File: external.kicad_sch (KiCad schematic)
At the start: 47 parts, among them J5 Keyboard Connector, J6 Joystick 1, J7 Joystick 2, Q7 BC547B, Q8 BC547B, U66 SN74ALS175N (КР1533ТМ8), U67 8282 (КР580ИР82), U68 КР556РТ2, U72 КР556РТ2, U73 SN74ALS08 (КР1533ЛИ1), U74 SN74ALS08 (КР1533ЛИ1)

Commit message: Version 1.0 schematics and PCB complete
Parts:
- D1, D10, D14, D15, D16, D17, D18, D19, D2, D20, D21, D22, D23, D24, D25, D26, D27, D28, D29, D3, D4, D5, D6, D7, D8, D9: symbol Device:D -> Delta_s_m_Lib:D
- DA1: symbol Device:R_Network09 -> Delta_s_m_Lib:R_Network09
- J5: symbol Connector_Generic:Conn_02x12_Odd_Even -> Delta_s_m_Lib:Conn_02x12_Odd_Even
- J6, J7: symbol Connector:DIN-7 -> Delta_s_m_Lib:DIN-7
- Q7, Q8: symbol Transistor_BJT:BC547 -> Delta_s_m_Lib:BC547
- R50, R51, R52, R54, R55, R56, R57, R58, R59: symbol Device:R -> Delta_s_m_Lib:R
- U66: symbol 74xx:74LS175 -> Delta_s_m_Lib:74LS175
- U67: symbol w_connectors:8282 (КР580ИР82) -> Delta_s_m_Lib:8282 (КР580ИР82)
- U68, U72: symbol w_connectors:КР556РТ2 -> Delta_s_m_Lib:КР556РТ2
- U73, U74: symbol 74xx:74LS08 -> Delta_s_m_Lib:74LS08

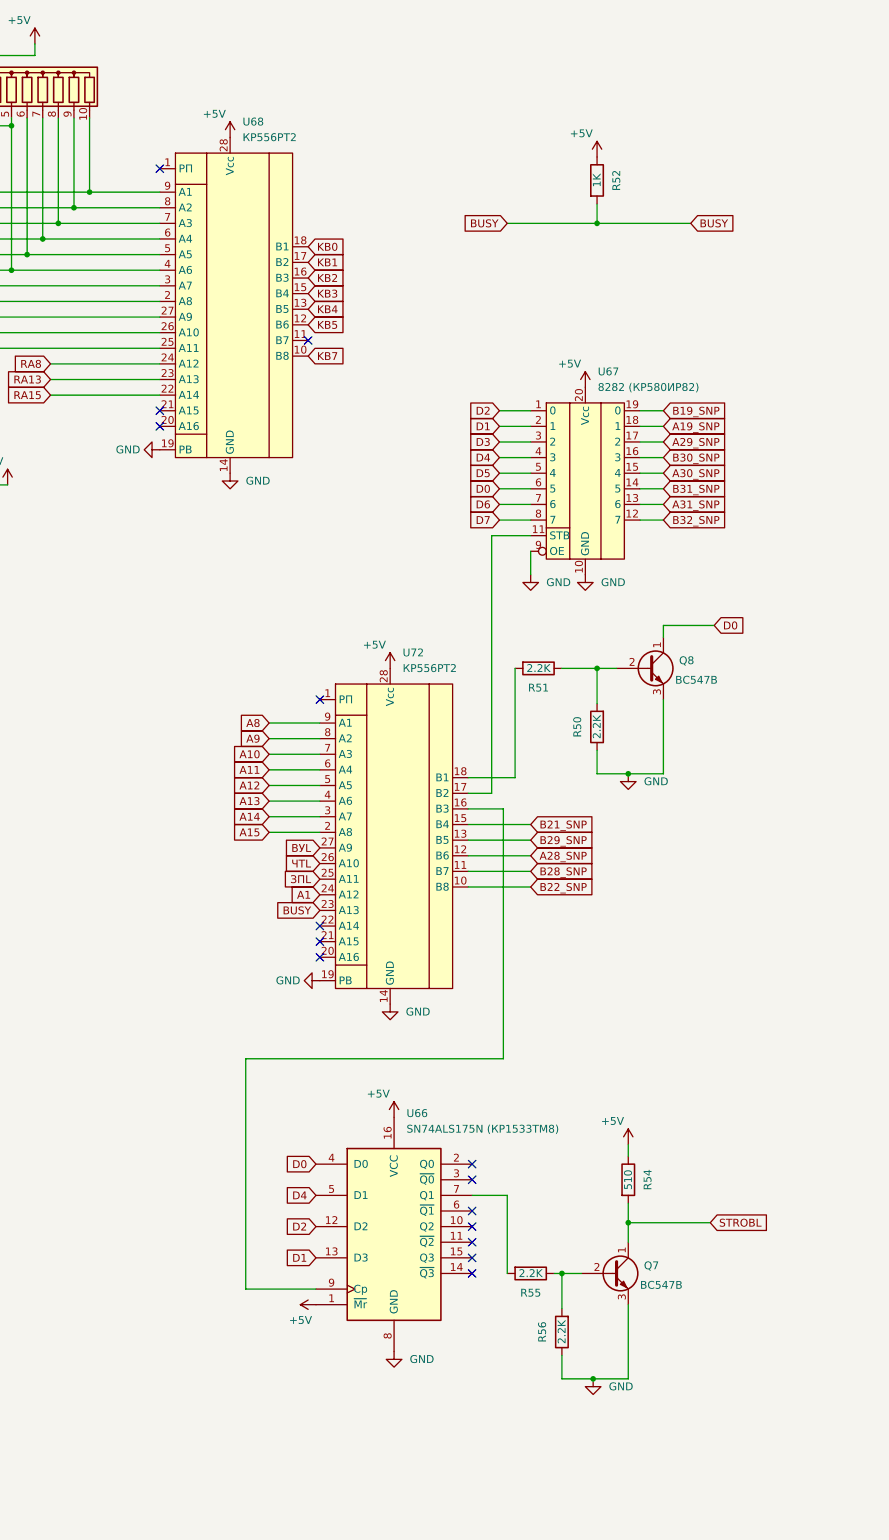
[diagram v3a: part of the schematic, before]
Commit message: Version 1.2 update
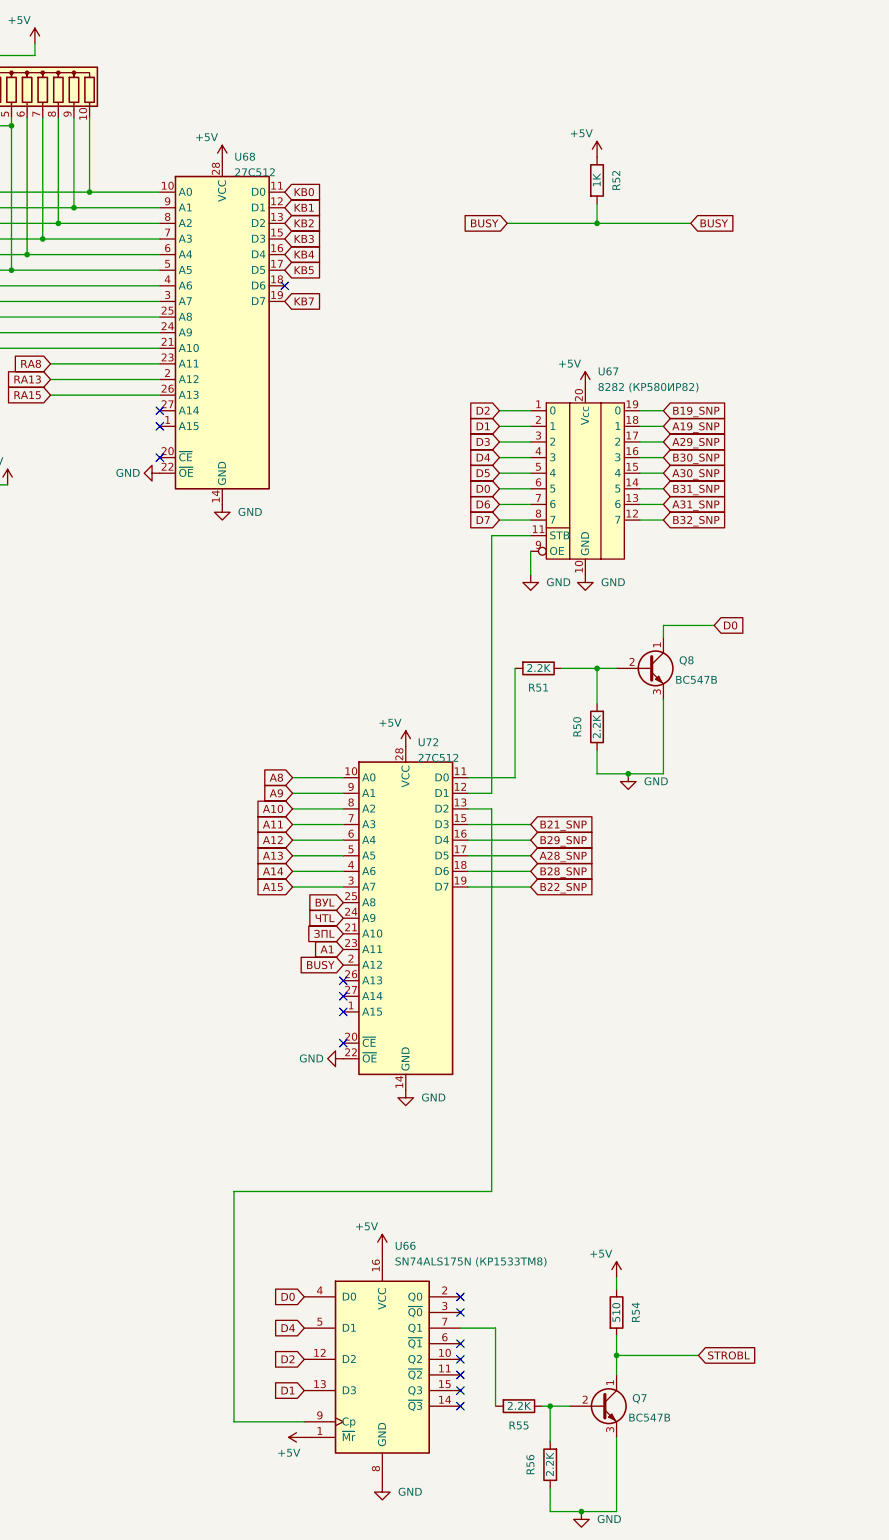
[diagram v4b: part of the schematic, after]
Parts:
- removed U68, U72: КР556РТ2, Package_DIP:DIP-28_W15.24mm_Socket, symbol Delta_s_m_Lib:КР556РТ2
- added U68, U72: 27C512, Delta_s_m_lib:DIP-28_W15.24mm_Socket, symbol Memory_EPROM:27C512
- D1, D10, D14, D15, D16, D17, D18, D19, D2, D20, D21, D22, D23, D24, D25, D26, D27, D28, D29, D3, D4, D5, D6, D7, D8, D9: footprint Diode_THT:D_DO-35_SOD27_P10.16mm_Horizontal -> Delta_sm_lib:D_DO-35_SOD27_P10.16mm_Horizontal
- DA1: footprint Resistor_THT:R_Array_SIP10 -> Delta_sm_lib:R_Array_SIP10
- J5: footprint Connector_IDC:IDC-Header_2x12_P2.54mm_Vertical -> Delta_sm_lib:IDC-Header_2x12_P2.54mm_Vertical
- J6, J7: footprint w_conn_av:DIN-7-Variable -> Delta_sm_lib:DIN-7-Variable
- Q7, Q8: footprint Package_TO_SOT_THT:TO-92_Inline -> Delta_sm_lib:TO-92_Inline
- R50, R51, R52, R54, R55, R56, R57, R58, R59: footprint Resistor_THT:R_Axial_DIN0207_L6.3mm_D2.5mm_P10.16mm_Horizontal -> Delta_sm_lib:R_Axial_DIN0207_L6.3mm_D2.5mm_P10.16mm_Horizontal
- U66: footprint Package_DIP:DIP-16_W7.62mm_Socket -> Delta_sm_lib:DIP-16_W7.62mm_Socket
- U67: footprint Package_DIP:DIP-20_W7.62mm_Socket -> Delta_sm_lib:DIP-20_W7.62mm_Socket
- U73, U74: footprint Package_DIP:DIP-14_W7.62mm_Socket -> Delta_sm_lib:DIP-14_W7.62mm_Socket
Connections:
- net +5V: now also U68.28 (VCC), U72.28 (VCC)
- net A1: now also U72.23 (A11)
- net A10: now also U72.8 (A2)
- net A11: now also U72.7 (A3)
- net A12: now also U72.6 (A4)
- net A13: now also U72.5 (A5)
- net A14: now also U72.4 (A6)
- net A15: now also U72.3 (A7)
- net A28_SNP: now also U72.17 (D5)
- net A8: now also U72.10 (A0)
- net A9: now also U72.9 (A1)
- net B21_SNP: now also U72.15 (D3)
- net B22_SNP: now also U72.19 (D7)
- net B28_SNP: now also U72.18 (D6)
- net B29_SNP: now also U72.16 (D4)
- net BUSY: now also U72.2 (A12)
- net GND: now also U68.14 (GND), U68.22 (~{OE}), U72.14 (GND), U72.22 (~{OE})
- net JOY3: now also U68.24 (A9)
- net JOY4: now also U68.25 (A8)
- net JOY5: now also U68.3 (A7)
- net JOY6: now also U68.4 (A6)
- net JOY7: now also U68.5 (A5)
- net KB0: now also U68.11 (D0)
- net KB1: now also U68.12 (D1)
- net KB2: now also U68.13 (D2)
- net KB3: now also U68.15 (D3)
- net KB4: now also U68.16 (D4)
- net KB5: now also U68.17 (D5)
- net KB7: now also U68.19 (D7)
- net KBD10: now also U68.8 (A2)
- net KBD11: now also U68.9 (A1)
- net KBD12: now also U68.10 (A0)
- net KBD2: now also U68.21 (A10)
- net KBD8: now also U68.6 (A4)
- net KBD9: now also U68.7 (A3)
- net RA13: now also U68.2 (A12)
- net RA15: now also U68.26 (A13)
- net RA8: now also U68.23 (A11)
- net ВУL: now also U72.25 (A8)
- net ЗПL: now also U72.21 (A10)
- net ЧТL: now also U72.24 (A9)
- net at U66.9 (Cp): now also U72.13 (D2)
- net at U67.11 (STB): now also U72.12 (D1)
- net at R51.2: now also U72.11 (D0)
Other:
- moved on the sheet: Q7, R54, R55, R56, U66

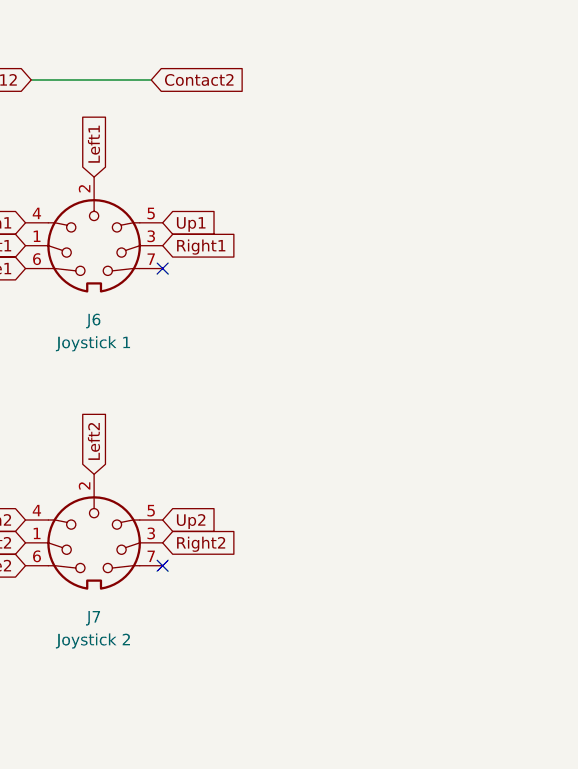
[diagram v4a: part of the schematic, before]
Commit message: Update 1.2, additional pins
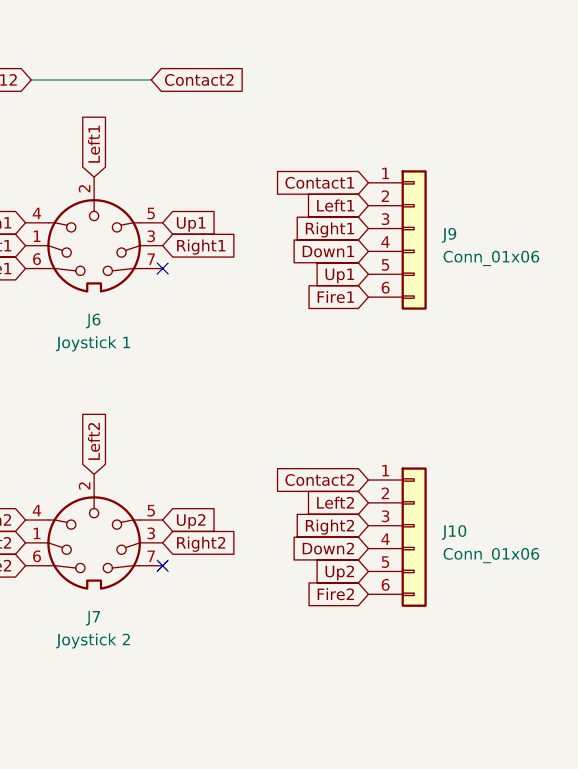
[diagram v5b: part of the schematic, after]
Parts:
- added J10, J9: Conn_01x06, Connector_PinHeader_2.54mm:PinHeader_1x06_P2.54mm_Vertical, symbol Connector_Generic:Conn_01x06
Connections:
- net Contact1: now also J9.1 (Pin_1)
- net Contact2: now also J10.1 (Pin_1)
- net Down1: now also J9.4 (Pin_4)
- net Down2: now also J10.4 (Pin_4)
- net Fire1: now also J9.6 (Pin_6)
- net Fire2: now also J10.6 (Pin_6)
- net Left1: now also J9.2 (Pin_2)
- net Left2: now also J10.2 (Pin_2)
- net Right1: now also J9.3 (Pin_3)
- net Right2: now also J10.3 (Pin_3)
- net Up1: now also J9.5 (Pin_5)
- net Up2: now also J10.5 (Pin_5)
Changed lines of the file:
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@@
+    )
+  )
+  (global_label "Down1" (shape input) (at 368.935 193.675 180) (fields_autoplaced)
+    (effects (font (size 1.27 1.27)) (justify right))
+    (property "Intersheetrefs" "${INTERSHEET_REFS}" (at 360.4138 193.5956 0)
+      (effects (font (size 1.27 1.27)) (justify right) hide)
     )
   )
@@
     )
   )
+  (global_label "Down2" (shape input) (at 368.935 226.695 180) (fields_autoplaced)
+    (effects (font (size 1.27 1.27)) (justify right))
+    (property "Intersheetrefs" "${INTERSHEET_REFS}" (at 360.4138 226.6156 0)
+      (effects (font (size 1.27 1.27)) (justify right) hide)
+    )
+  )
   (global_label "KBD16" (shape input) (at 108.585 134.62 0) (fields_autoplaced)
     (effects (font (size 1.27 1.27)) (justify left))
@@
     )
   )
+  (global_label "Contact1" (shape input) (at 368.935 186.055 180) (fields_autoplaced)
+    (effects (font (size 1.27 1.27)) (justify right))
+    (property "Intersheetrefs" "${INTERSHEET_REFS}" (at 358.0552 185.9756 0)
+      (effects (font (size 1.27 1.27)) (justify right) hide)
+    )
+  )
   (global_label "Up2" (shape input) (at 343.535 152.4 0) (fields_autoplaced)
     (effects (font (size 1.27 1.27)) (justify left))
@@
     )
   )
+  (global_label "Contact2" (shape input) (at 368.935 219.075 180) (fields_autoplaced)
+    (effects (font (size 1.27 1.27)) (justify right))
+    (property "Intersheetrefs" "${INTERSHEET_REFS}" (at 358.0552 218.9956 0)
+      (effects (font (size 1.27 1.27)) (justify right) hide)
+    )
+  )
   (global_label "KBD12" (shape input) (at 344.17 40.64 0) (fields_autoplaced)
     (effects (font (size 1.27 1.27)) (justify left))
@@
     )
   )
+  (global_label "Left1" (shape input) (at 368.935 188.595 180) (fields_autoplaced)
+    (effects (font (size 1.27 1.27)) (justify right))
+    (property "Intersheetrefs" "${INTERSHEET_REFS}" (at 361.2516 188.595 0)
+      (effects (font (size 1.27 1.27)) (justify right) hide)
+    )
+  )
   (global_label "KBD10" (shape input) (at 344.17 38.1 0) (fields_autoplaced)
     (effects (font (size 1.27 1.27)) (justify left))
@@
     )
   )
+  (global_label "Right2" (shape input) (at 368.935 224.155 180) (fields_autoplaced)
+    (effects (font (size 1.27 1.27)) (justify right))
+    (property "Intersheetrefs" "${INTERSHEET_REFS}" (at 359.9212 224.155 0)
+      (effects (font (size 1.27 1.27)) (justify right) hide)
+    )
+  )
   (global_label "D7" (shape input) (at 236.855 97.155 180) (fields_autoplaced)
     (effects (font (size 1.27 1.27)) (justify right))
@@
     )
   )
+  (global_label "Up1" (shape input) (at 368.935 196.215 180) (fields_autoplaced)
+    (effects (font (size 1.27 1.27)) (justify right))
+    (property "Intersheetrefs" "${INTERSHEET_REFS}" (at 362.3402 196.215 0)
+      (effects (font (size 1.27 1.27)) (justify right) hide)
+    )
+  )
   (global_label "JOY7" (shape input) (at 324.485 116.84 180) (fields_autoplaced)
     (effects (font (size 1.27 1.27)) (justify right))
@@
     )
   )
+  (global_label "Fire2" (shape input) (at 368.935 231.775 180) (fields_autoplaced)
+    (effects (font (size 1.27 1.27)) (justify right))
+    (property "Intersheetrefs" "${INTERSHEET_REFS}" (at 361.7443 231.6956 0)
+      (effects (font (size 1.27 1.27)) (justify right) hide)
+    )
+  )
   (global_label "KBD15" (shape input) (at 108.585 144.145 0) (fields_autoplaced)
     (effects (font (size 1.27 1.27)) (justify left))
@@
     )
   )
+  (global_label "Fire1" (shape input) (at 368.935 198.755 180) (fields_autoplaced)
+    (effects (font (size 1.27 1.27)) (justify right))
+    (property "Intersheetrefs" "${INTERSHEET_REFS}" (at 361.7443 198.6756 0)
+      (effects (font (size 1.27 1.27)) (justify right) hide)
+    )
+  )
   (global_label "D2" (shape input) (at 205.105 233.68 180) (fields_autoplaced)
     (effects (font (size 1.27 1.27)) (justify right))
@@
     )
   )
+  (global_label "Left2" (shape input) (at 368.935 221.615 180) (fields_autoplaced)
+    (effects (font (size 1.27 1.27)) (justify right))
+    (property "Intersheetrefs" "${INTERSHEET_REFS}" (at 361.2516 221.615 0)
+      (effects (font (size 1.27 1.27)) (justify right) hide)
+    )
+  )
   (global_label "Fire1" (shape input) (at 343.535 116.84 0) (fields_autoplaced)
     (effects (font (size 1.27 1.27)) (justify left))
@@
     )
   )
+  (global_label "Up2" (shape input) (at 368.935 229.235 180) (fields_autoplaced)
+    (effects (font (size 1.27 1.27)) (justify right))
+    (property "Intersheetrefs" "${INTERSHEET_REFS}" (at 362.3402 229.235 0)
+      (effects (font (size 1.27 1.27)) (justify right) hide)
+    )
+  )
   (global_label "KB2" (shape input) (at 201.93 48.895 0) (fields_autoplaced)
     (effects (font (size 1.27 1.27)) (justify left))
@@
     (effects (font (size 1.27 1.27)) (justify right))
     (property "Intersheetrefs" "${INTERSHEET_REFS}" (at 317.4757 97.7106 0)
+      (effects (font (size 1.27 1.27)) (justify right) hide)
+    )
+  )
+  (global_label "Right1" (shape input) (at 368.935 191.135 180) (fields_autoplaced)
+    (effects (font (size 1.27 1.27)) (justify right))
+    (property "Intersheetrefs" "${INTERSHEET_REFS}" (at 359.9212 191.135 0)
       (effects (font (size 1.27 1.27)) (justify right) hide)
     )
@@
         (path "/85193df6-d35d-456e-b7a4-64fabf18f664"
           (reference "#PWR0253") (unit 1)
+        )
+      )
+    )
+  )
+  (symbol (lib_id "Connector_Generic:Conn_01x06") (at 374.015 224.155 0) (unit 1)
+    (in_bom yes) (on_board yes) (dnp no) (fields_autoplaced)
+    (property "Reference" "J10" (at 377.19 224.79 0)
+      (effects (font (size 1.27 1.27)) (justify left))
+    )
+    (property "Value" "Conn_01x06" (at 377.19 227.33 0)
+      (effects (font (size 1.27 1.27)) (justify left))
+    )
+    (property "Footprint" "Connector_PinHeader_2.54mm:PinHeader_1x06_P2.54mm_Vertical" (at 374.015 224.155 0)
+      (effects (font (size 1.27 1.27)) hide)
+    )
+    (property "Datasheet" "~" (at 374.015 224.155 0)
+      (effects (font (size 1.27 1.27)) hide)
+    )
+    (pin "1")
+    (pin "2")
+    (pin "3")
+    (pin "4")
+    (pin "5")
+    (pin "6")
+    (instances
+      (project "delta48m"
+        (path "/31325de8-16cf-4c6f-92cf-6f5a8aaa6830/b0522bc4-51ff-4c7a-805e-784ede031ae9"
+          (reference "J10") (unit 1)
         )
       )
@@
         )
       )
+    )
+  )
+  (symbol (lib_id "Connector_Generic:Conn_01x06") (at 374.015 191.135 0) (unit 1)
+    (in_bom yes) (on_board yes) (dnp no) (fields_autoplaced)
+    (property "Reference" "J9" (at 377.19 191.77 0)
+      (effects (font (size 1.27 1.27)) (justify left))
+    )
+    (property "Value" "Conn_01x06" (at 377.19 194.31 0)
+      (effects (font (size 1.27 1.27)) (justify left))
+    )
+    (property "Footprint" "Connector_PinHeader_2.54mm:PinHeader_1x06_P2.54mm_Vertical" (at 374.015 191.135 0)
+      (effects (font (size 1.27 1.27)) hide)
+    )
+    (property "Datasheet" "~" (at 374.015 191.135 0)
+      (effects (font (size 1.27 1.27)) hide)
+    )
+    (pin "1")
+    (pin "2")
+    (pin "3")
+    (pin "4")
+    (pin "5")
+    (pin "6")
+    (instances
+      (project "delta48m"
+        (path "/31325de8-16cf-4c6f-92cf-6f5a8aaa6830/b0522bc4-51ff-4c7a-805e-784ede031ae9"
+          (reference "J9") (unit 1)
+        )
+      )
